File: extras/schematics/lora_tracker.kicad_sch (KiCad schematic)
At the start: 29 parts, among them J1 ANT, J4 Conn_01x03_Female, SW1 SW_Push, SW2 EC11, U1 ESP32, U2 E22-400M30S, U3 RA-01, U4 INP441, U5 MAX98357A, U6 SSD1306, U7 ATGM336H

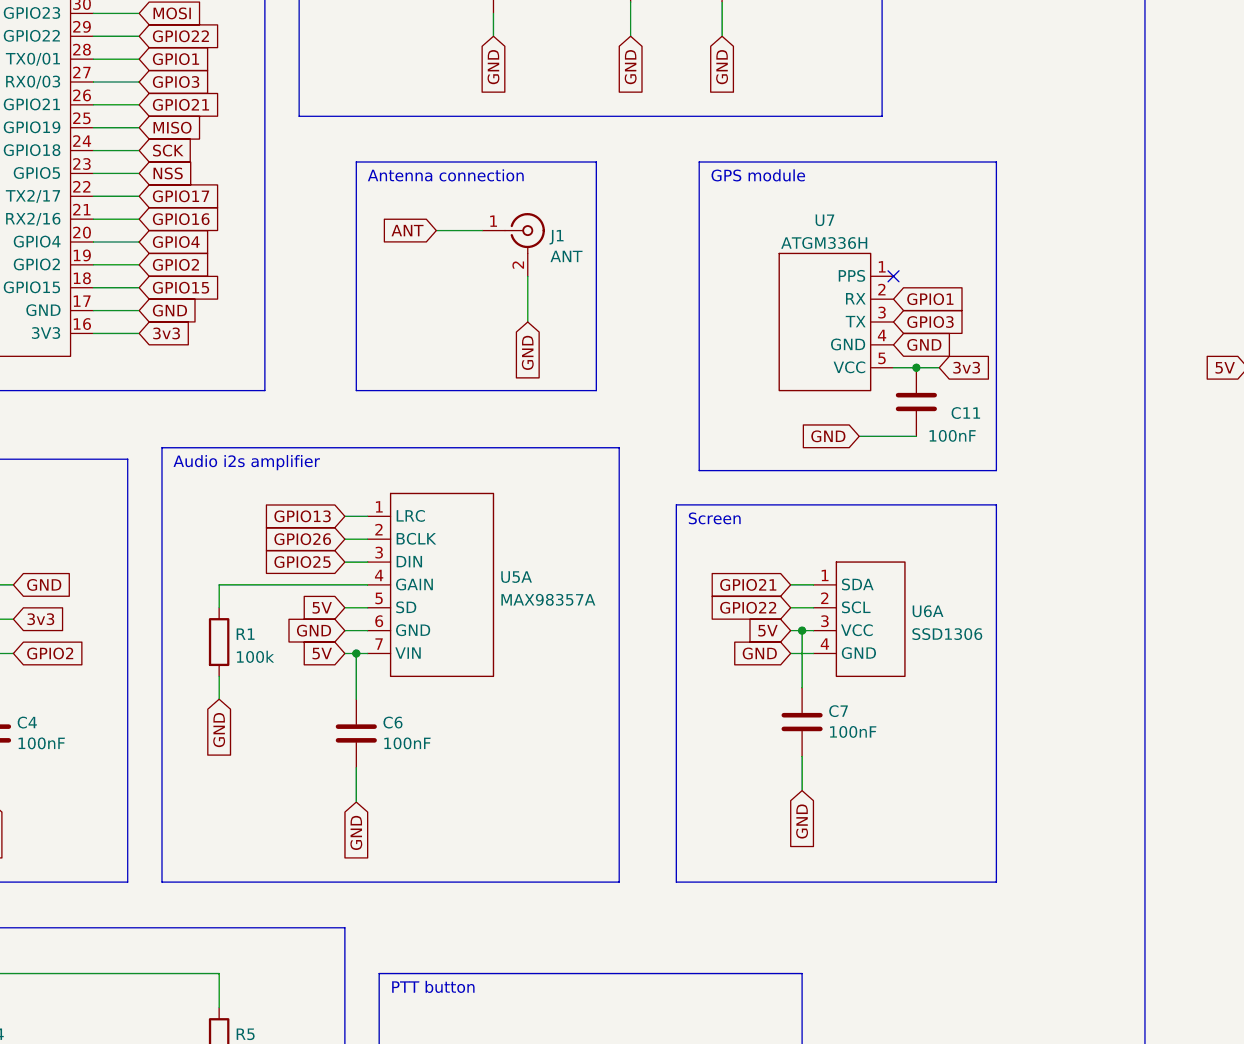
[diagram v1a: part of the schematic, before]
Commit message: Update schematics
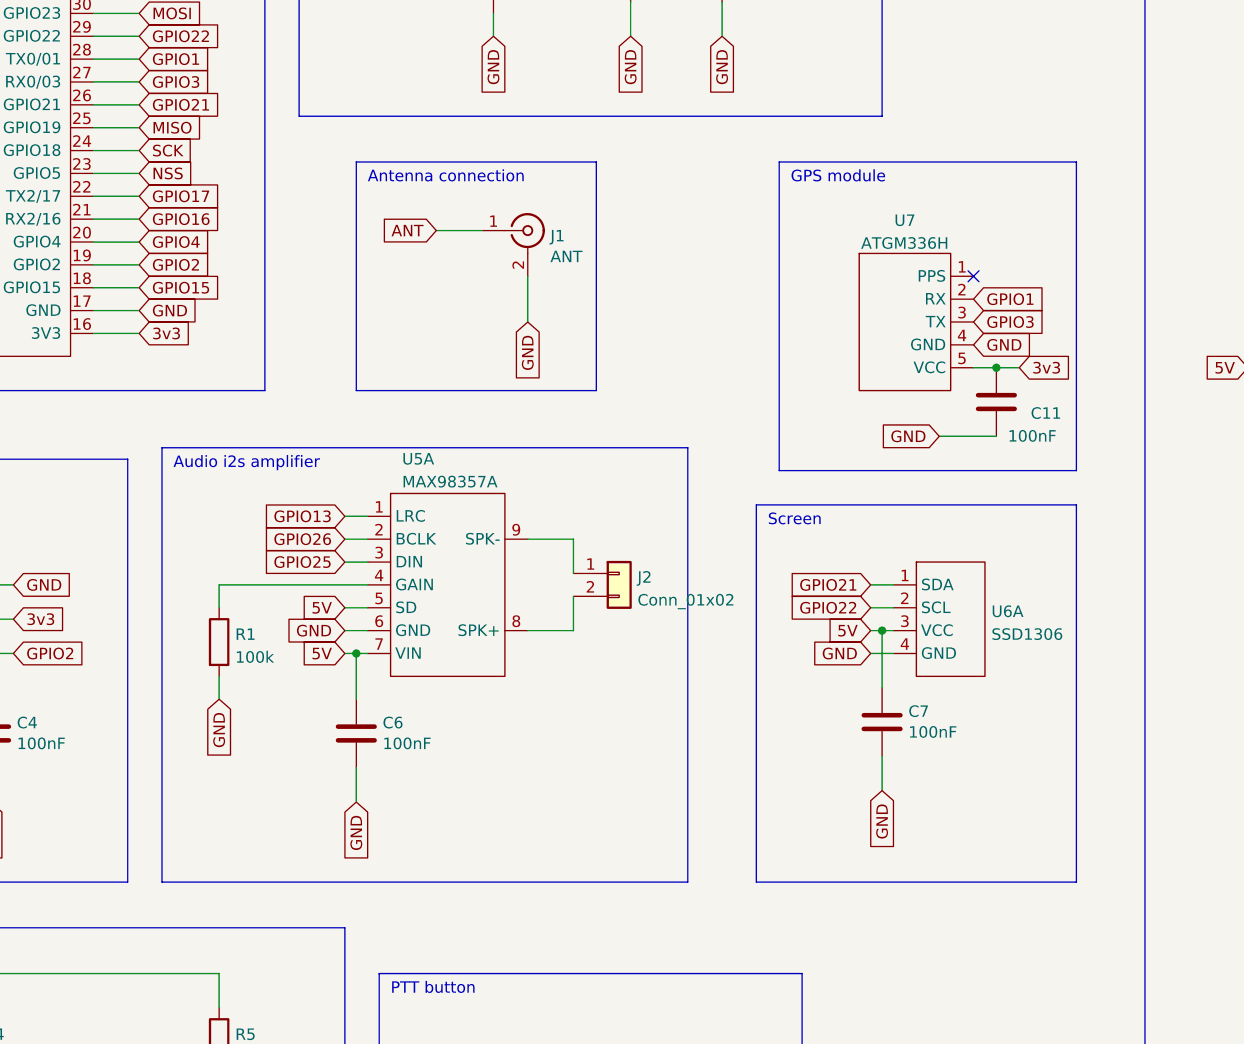
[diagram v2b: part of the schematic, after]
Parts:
- added J2: Conn_01x02, Connector_PinHeader_2.54mm:PinHeader_2x01_P2.54mm_Vertical_SMD, symbol Connector_Generic:Conn_01x02
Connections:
- new net: J2.1 (Pin_1), U5.9 (SPK-)
- new net: J2.2 (Pin_2), U5.8 (SPK+)
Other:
- moved on the sheet: C11, C7, U6A, U7
